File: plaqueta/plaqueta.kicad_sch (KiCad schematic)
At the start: 9 parts, among them J1 Conn_01x08_Female, J2 Conn_01x04_Female, J3 POWER, J4 BORN_RELAY, K1 FINDER-36.11, Q1 BC337, U1 ESP32_DevKit_V1_DOIT

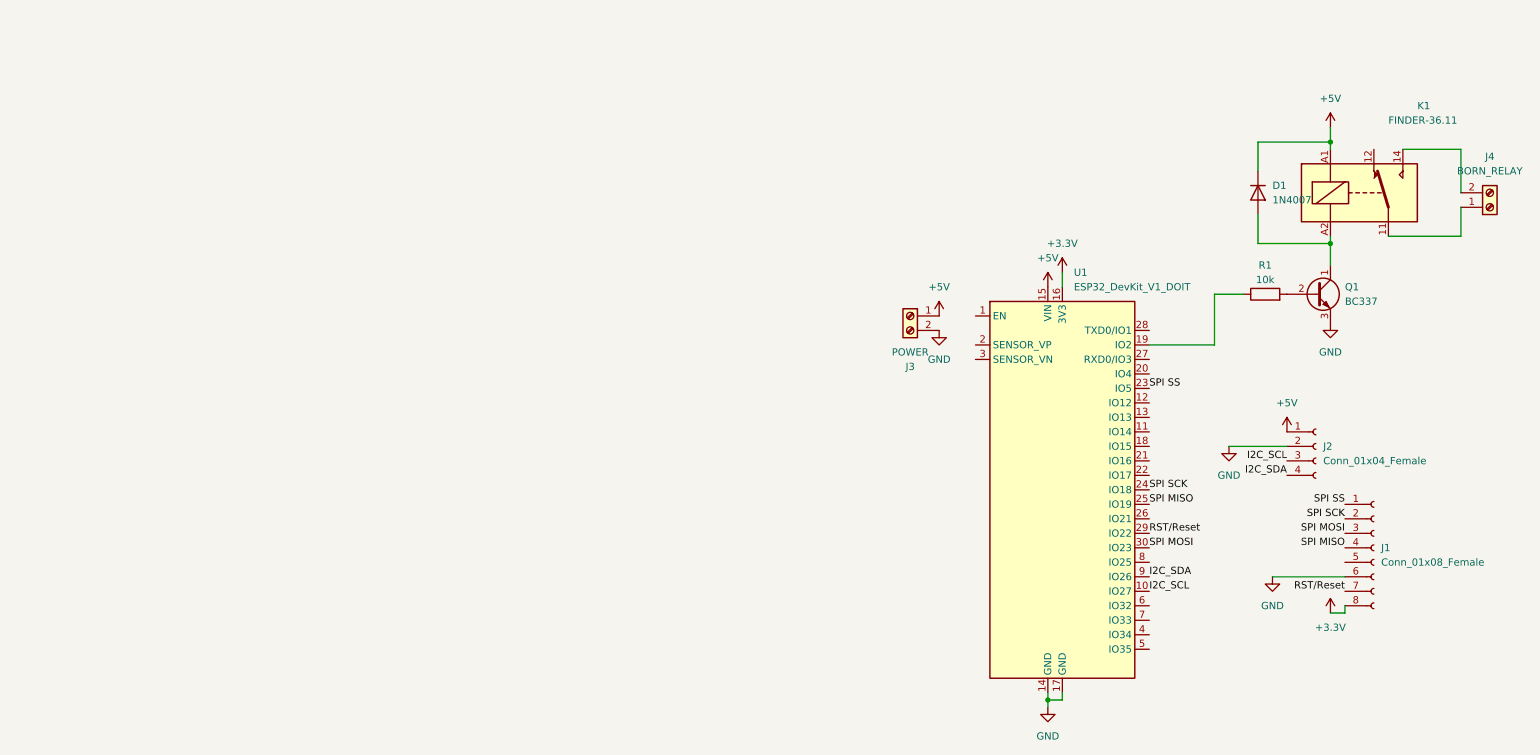
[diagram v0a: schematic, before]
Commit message: actualizado el informe
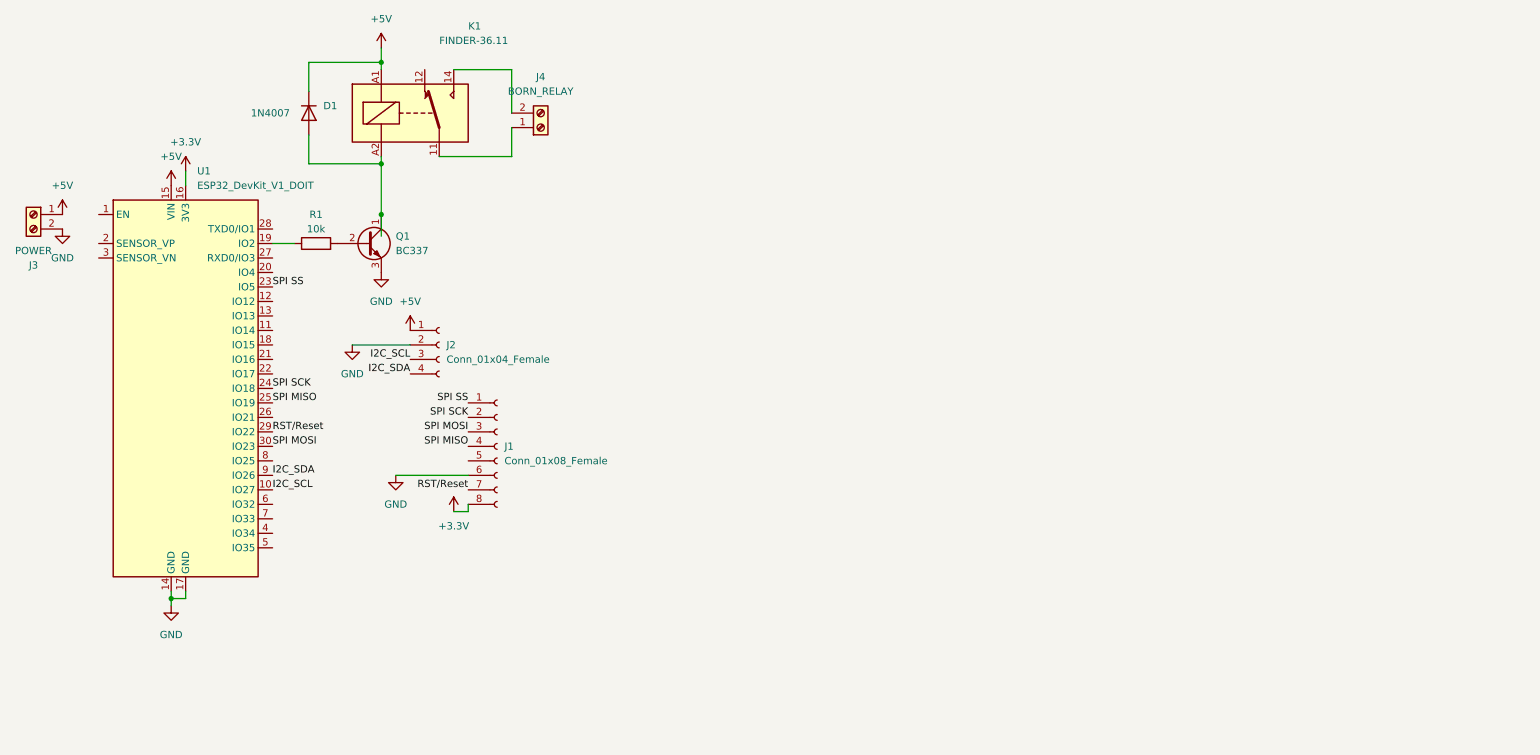
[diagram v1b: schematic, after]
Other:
- moved on the sheet: D1, J1, J2, J3, J4, K1, Q1, R1, U1
